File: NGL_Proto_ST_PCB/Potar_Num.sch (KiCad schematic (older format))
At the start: 3 parts, among them U10 10K, U11 20k

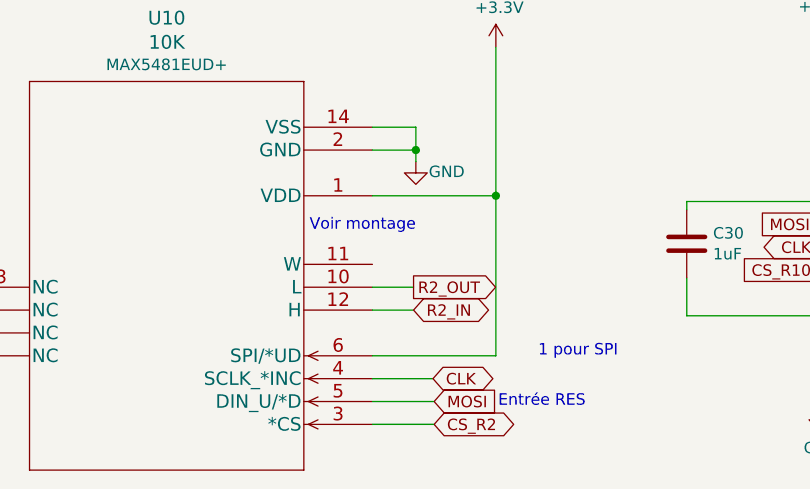
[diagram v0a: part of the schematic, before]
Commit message: Avancement après réunion mercredi
finir pour mettre en review puis attente.
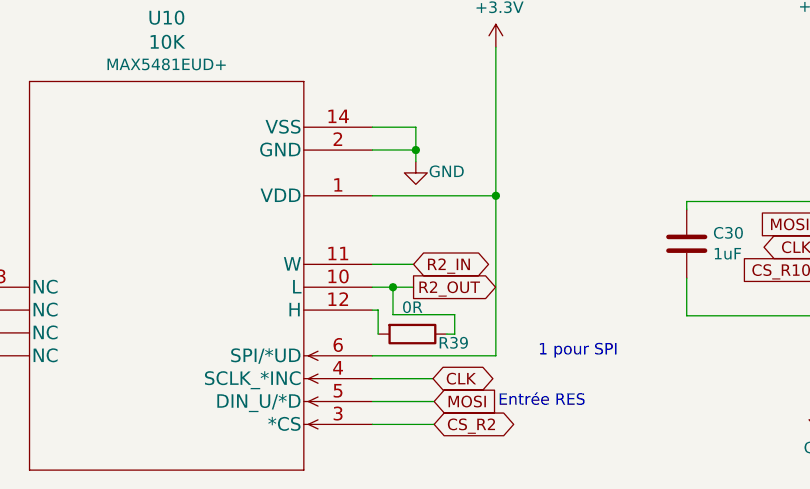
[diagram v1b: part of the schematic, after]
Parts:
- added R39: 0R, Resistor_SMD:R_0805_2012Metric, symbol Device:R
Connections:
- net R2_IN: now also U10.11 (W); no longer U10.12 (H)
- net R2_OUT: now also R39.1
- new net: R39.2, U10.12 (H)
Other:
- note removed: "Voir montage"
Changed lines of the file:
@@
 Text Notes 5260 5230 0    50   ~ 0
 Entrée RES
-Text GLabel 4890 4800 2    50   BiDi ~ 0
+Text GLabel 4890 4600 2    50   BiDi ~ 0
 R2_IN
 Text GLabel 4890 4700 2    50   Output ~ 0
@@
 Wire Wire Line
 	4710 5100 4975 5100
-Wire Wire Line
-	4890 4800 4710 4800
-Wire Wire Line
-	4890 4700 4710 4700
-Text Notes 4435 4460 0    50   ~ 0
-Voir montage
 $Comp
 L power:+3.3V #PWR040
@@
 Wire Wire Line
 	4900 4100 4900 4150
+$Comp
+L Device:R R39
+U 1 1 62A152EA
+P 4885 4905
+F 0 "R39" V 4925 5085 50  0000 C CNN
+F 1 "0R" V 4769 4905 50  0000 C CNN
+F 2 "Resistor_SMD:R_0805_2012Metric" V 4815 4905 50  0001 C CNN
+F 3 "~" H 4885 4905 50  0001 C CNN
+	1    4885 4905
+	0    1    1    0
+$EndComp
+Wire Wire Line
+	4890 4700 4800 4700
+Wire Wire Line
+	4890 4600 4710 4600
+Wire Wire Line
+	4735 4905 4735 4800
+Wire Wire Line
+	4735 4800 4710 4800
+Wire Wire Line
+	5035 4905 5070 4905
+Wire Wire Line
+	5070 4905 5070 4820
+Wire Wire Line
+	5070 4820 4800 4820
+Wire Wire Line
+	4800 4820 4800 4700
+Connection ~ 4800 4700
+Wire Wire Line
+	4800 4700 4710 4700
 $EndSCHEMATC
